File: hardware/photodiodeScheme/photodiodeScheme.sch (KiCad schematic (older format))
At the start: 1 part

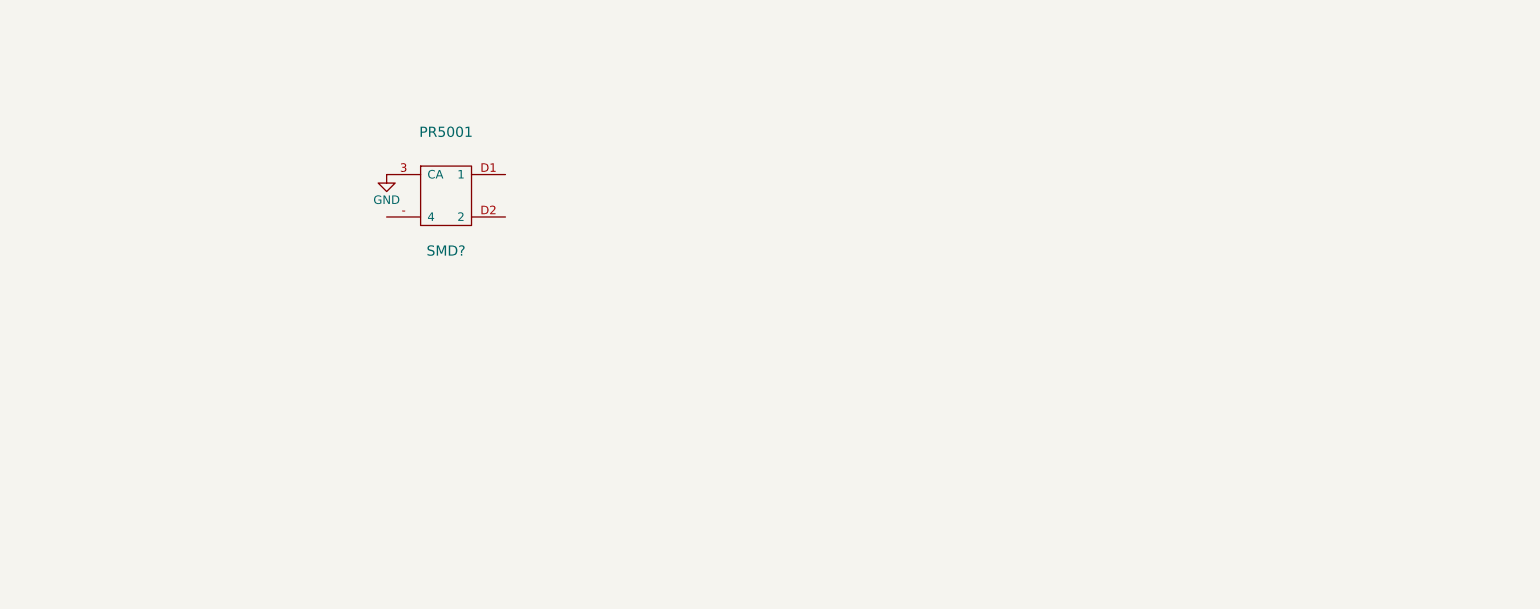
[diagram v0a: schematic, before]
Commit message: Add files via upload
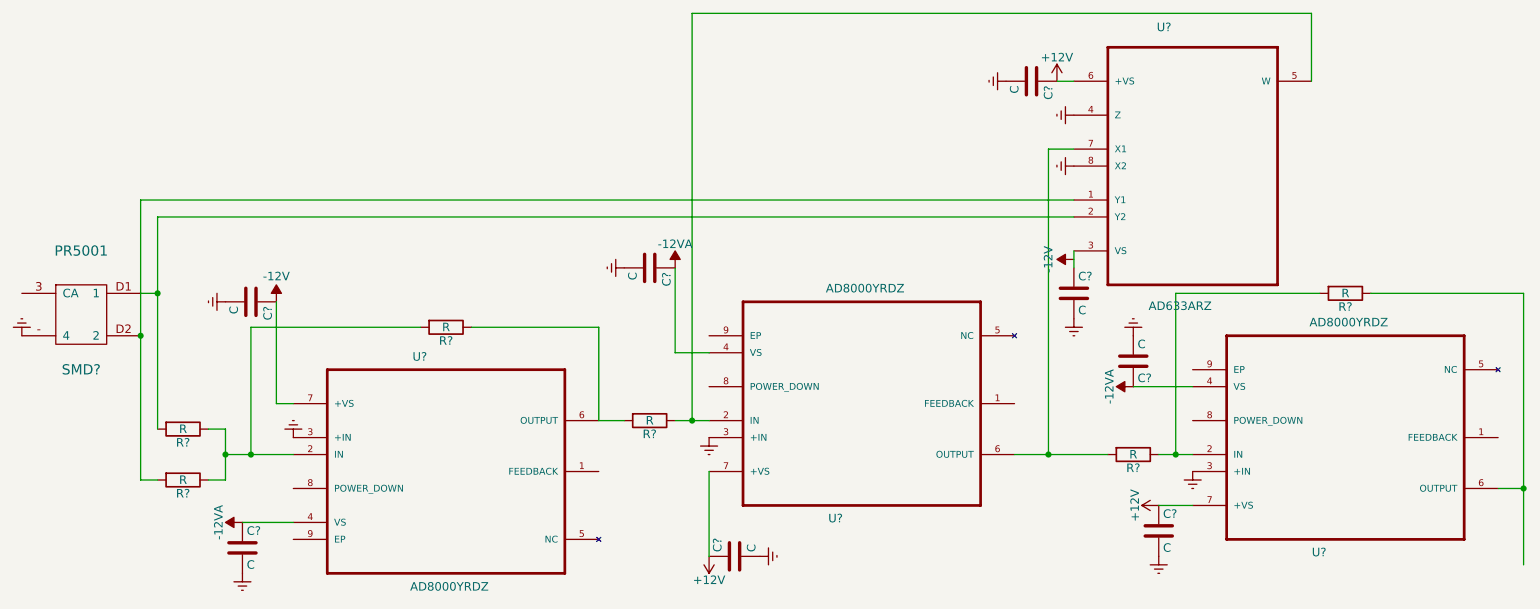
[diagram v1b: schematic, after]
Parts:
- removed SMD?: PR5001, symbol PR5001
- added C? (x8): C, symbol C
- added R? (x6): R, symbol R
- added SMD?: PR5001, symbol PR5001
- added U?: AD633ARZ, SOIC127P600X175-8N, symbol AD633ARZ
- added U? (x3): AD8000YRDZ, SOIC127P600X175-9N, symbol AD8000YRDZ
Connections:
- new net: R?.2, SMD?.D1 (1), U?.2 (Y2)
- new net: R?.2, SMD?.D2 (2), U?.1 (Y1)
- new net: C?.1, U?.3 (VS)
- new net: R?.1, U?.2 (IN), U?.5 (W)
- new net: R?.2, U?.6 (OUTPUT), U?.7 (X1)
- new net: R?.1, R?.1, R?.2, U?.2 (IN)
- new net: R?.1, R?.2, U?.6 (OUTPUT)
- new net: R?.1, R?.2, U?.2 (IN)
- new net: R?.1, U?.6 (OUTPUT)
- new net +12V: C?.1, C?.1, C?.1, U?.6 (+VS), U?.7 (+VS), U?.7 (+VS)
- new net -12V: C?.1, U?.7 (+VS)
- new net -12VA: C?.1, C?.1, C?.1, U?.4 (VS), U?.4 (VS), U?.4 (VS)
- new net Earth: C?.2, C?.2, C?.2, C?.2, C?.2, C?.2, C?.2, C?.2, SMD?.- (4), U?.3 (+IN), U?.3 (+IN), U?.3 (+IN), U?.4 (Z), U?.8 (X2)
